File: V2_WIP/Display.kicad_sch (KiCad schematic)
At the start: 13 parts, among them U11 *SN74LV1T34DBVRG4, U4 *HT16k33, U402 *KW4-804CGB, U5 *7seg_1x1_rgb, U6 *7seg_1x1_rgb, U7 *7seg_1x1_rgb

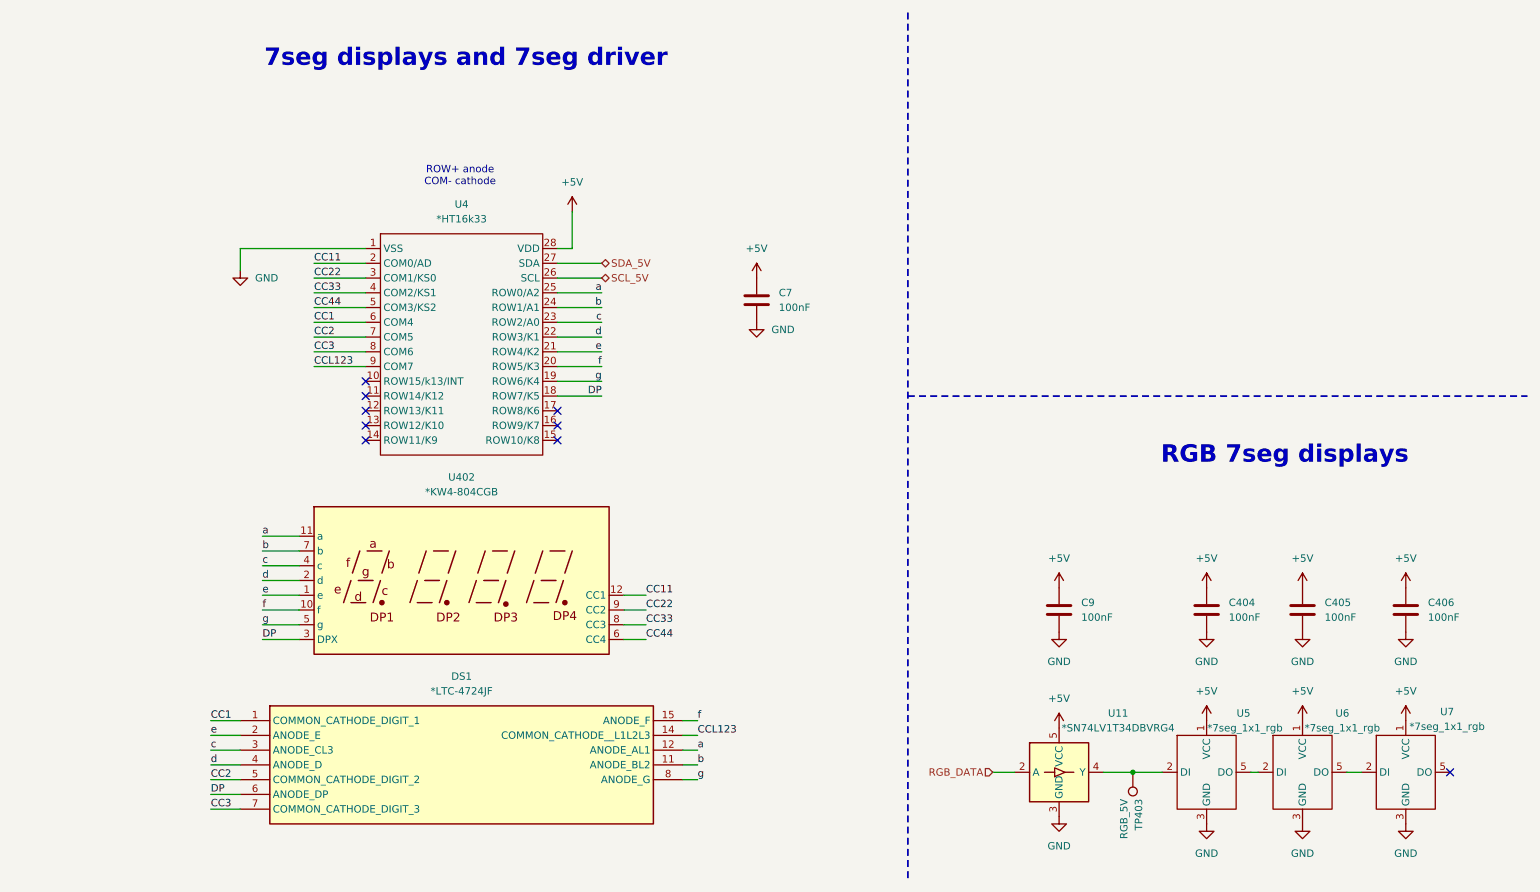
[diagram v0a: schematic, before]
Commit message: updated list of changes in README.md
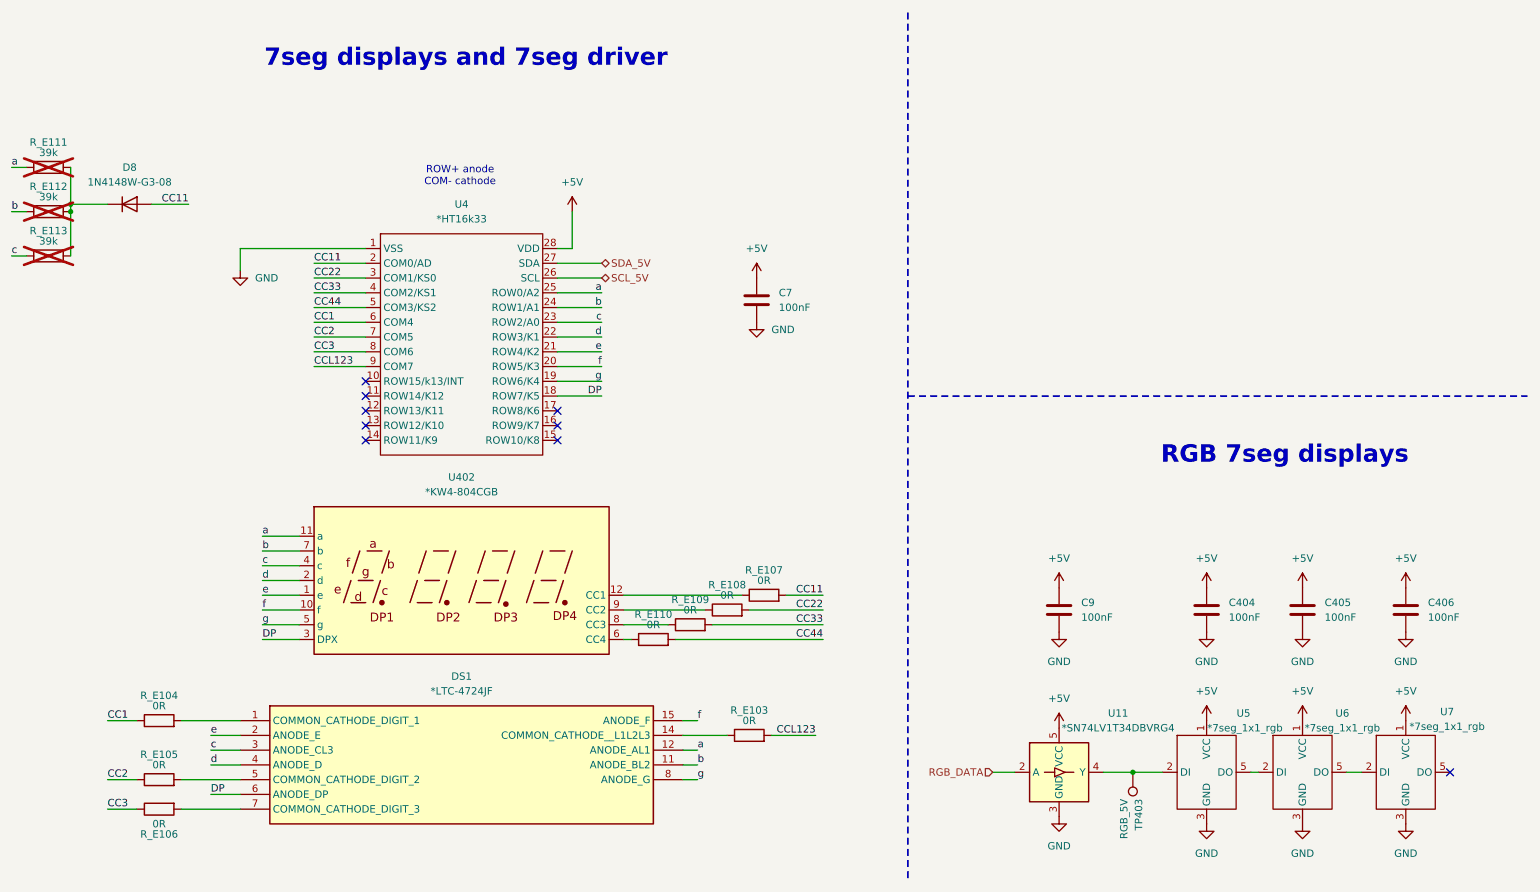
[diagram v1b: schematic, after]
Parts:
- added D8: 1N4148W-G3-08, Diode_SMD:D_SOD-123, symbol Device:D
- added R_E103, R_E104, R_E105, R_E106, R_E107, R_E108, R_E109, R_E110: 0R, Resistor_SMD:R_0603_1608Metric_Pad0.98x0.95mm_HandSolder, symbol Device:R
- added R_E111, R_E112, R_E113: 39k, Resistor_SMD:R_0603_1608Metric_Pad0.98x0.95mm_HandSolder, symbol Device:R
- TP403: footprint TestPoint:TestPoint_Pad_D1.5mm -> TestPoint:TestPoint_Pad_D1.0mm
- U4: footprint w_smd_dil:soic-28 -> Package_SO:SOIC-28W_7.5x17.9mm_P1.27mm
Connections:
- net CC1: now also R_E104.1; no longer DS1.1 (COMMON_CATHODE_DIGIT_1)
- net CC11: now also D8.2 (A), R_E107.2; no longer U402.12 (CC1)
- net CC2: now also R_E105.1; no longer DS1.5 (COMMON_CATHODE_DIGIT_2)
- net CC22: now also R_E108.2; no longer U402.9 (CC2)
- net CC3: now also R_E106.1; no longer DS1.7 (COMMON_CATHODE_DIGIT_3)
- net CC33: now also R_E109.2; no longer U402.8 (CC3)
- net CC44: now also R_E110.2; no longer U402.6 (CC4)
- net CCL123: now also R_E103.2; no longer DS1.14 (COMMON_CATHODE__L1L2L3)
- net a: now also R_E111.1
- net b: now also R_E112.1
- net c: now also R_E113.1
- new net: DS1.5 (COMMON_CATHODE_DIGIT_2), R_E105.2
- new net: DS1.1 (COMMON_CATHODE_DIGIT_1), R_E104.2
- new net: DS1.14 (COMMON_CATHODE__L1L2L3), R_E103.1
- new net: DS1.7 (COMMON_CATHODE_DIGIT_3), R_E106.2
- new net: R_E108.1, U402.9 (CC2)
- new net: R_E107.1, U402.12 (CC1)
- new net: R_E109.1, U402.8 (CC3)
- new net: D8.1 (K), R_E111.2, R_E112.2, R_E113.2
- new net: R_E110.1, U402.6 (CC4)
